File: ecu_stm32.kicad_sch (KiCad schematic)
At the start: 46 parts, among them J16 USB-C, J17 ARM Cortex Debug, Y2 16MHz

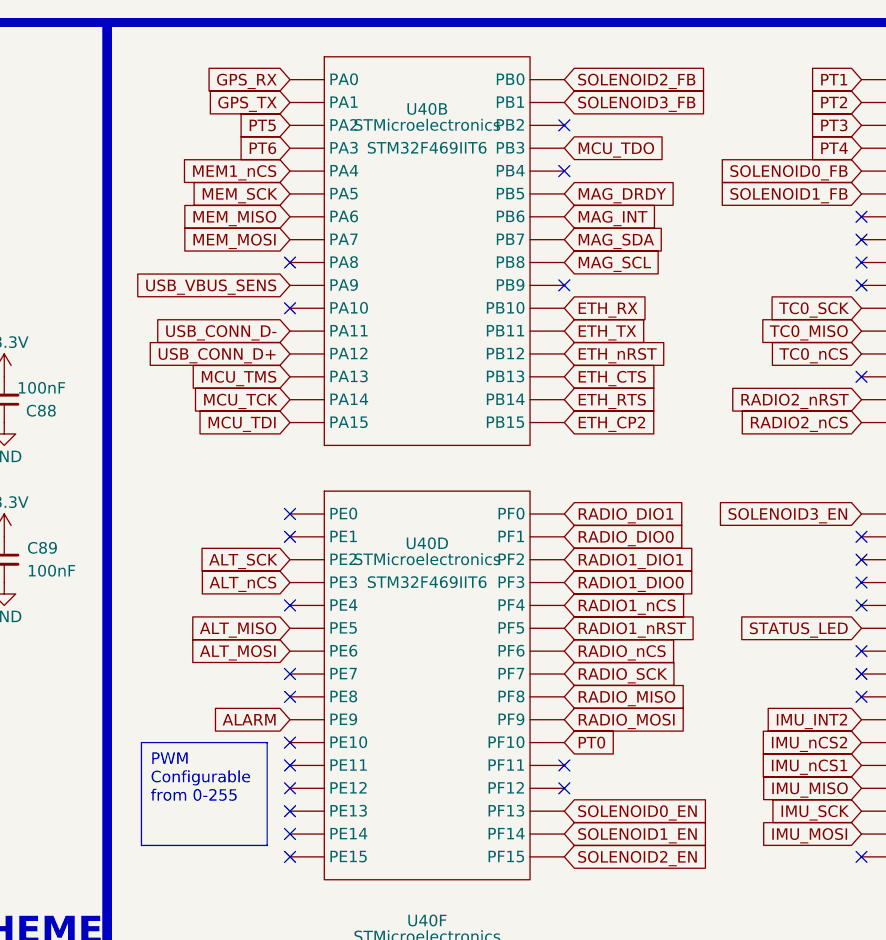
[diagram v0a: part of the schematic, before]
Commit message: Finished
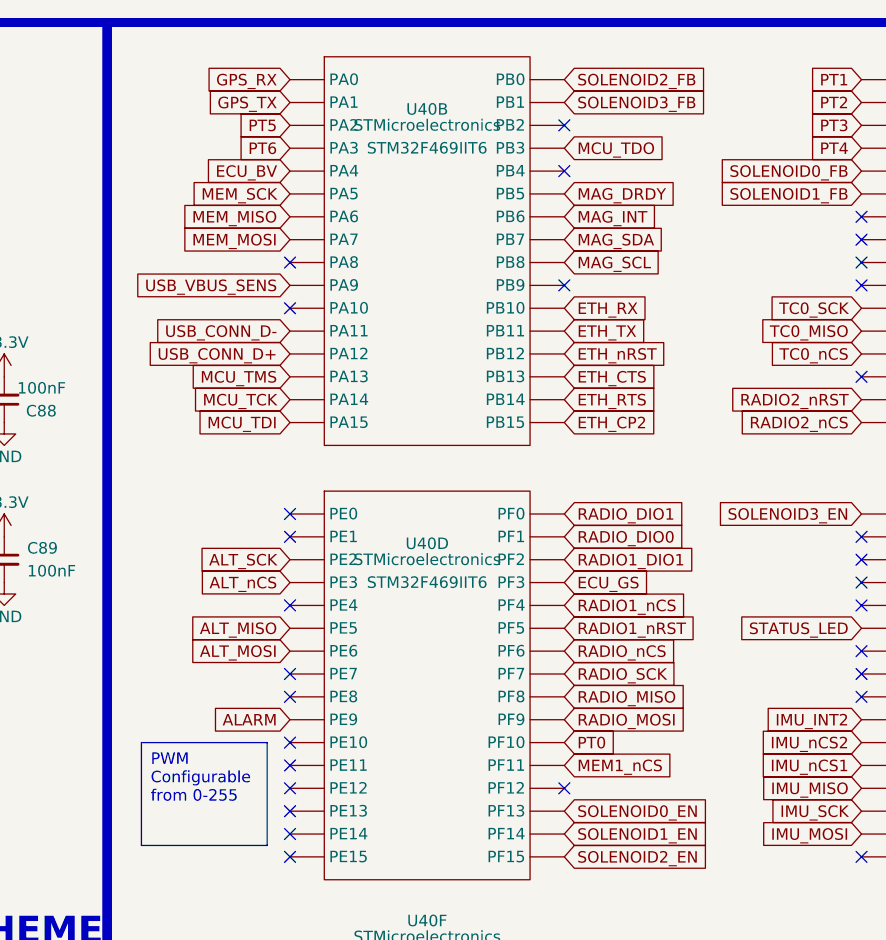
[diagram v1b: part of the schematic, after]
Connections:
- net MEM1_nCS: now also U40.59 (PF11); no longer U40.50 (PA4)
- net RADIO1_DIO0 renamed ECU_GS
- new net ECU_BV: U40.50 (PA4)
- no-connect marks 73 -> 72
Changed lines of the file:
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@@
 	)
 	(no_connect
-		(at 193.04 96.52)
-	)
-	(no_connect
 		(at 162.56 86.36)
 	)
@@
 		)
 	)
+	(global_label "ECU_GS"
+		(shape input)
+		(at 193.04 76.2 0)
+		(fields_autoplaced yes)
+		(effects
+			(font
+				(size 1.27 1.27)
+			)
+			(justify left)
+		)
+		(property "Intersheetrefs" "${INTERSHEET_REFS}"
+			(at 203.2218 76.2 0)
+			(effects
+				(font
+					(size 1.27 1.27)
+				)
+				(justify left)
+				(hide yes)
+			)
+		)
+	)
 	(global_label "IMU_MOSI"
 		(shape input)
@@
 		)
 	)
+	(global_label "ECU_BV"
+		(shape input)
+		(at 162.56 30.48 180)
+		(fields_autoplaced yes)
+		(effects
+			(font
+				(size 1.27 1.27)
+			)
+			(justify right)
+		)
+		(property "Intersheetrefs" "${INTERSHEET_REFS}"
+			(at 152.4991 30.48 0)
+			(effects
+				(font
+					(size 1.27 1.27)
+				)
+				(justify right)
+				(hide yes)
+			)
+		)
+	)
 	(global_label "PT4"
 		(shape input)
@@
 		)
 	)
-	(global_label "RADIO1_DIO0"
-		(shape input)
-		(at 193.04 76.2 0)
-		(fields_autoplaced yes)
-		(effects
-			(font
-				(size 1.27 1.27)
-			)
-			(justify left)
-		)
-		(property "Intersheetrefs" "${INTERSHEET_REFS}"
-			(at 208.181 76.2 0)
-			(effects
-				(font
-					(size 1.27 1.27)
-				)
-				(justify left)
-				(hide yes)
-			)
-		)
-	)
 	(global_label "GPS_INT"
 		(shape input)
@@
 		)
 	)
-	(global_label "MEM1_nCS"
+	(global_label "GPS_TX"
 		(shape input)
-		(at 162.56 30.48 180)
+		(at 162.56 22.86 180)
 		(fields_autoplaced yes)
 		(effects
@@
 		)
 		(property "Intersheetrefs" "${INTERSHEET_REFS}"
-			(at 149.7174 30.48 0)
+			(at 152.6806 22.86 0)
 			(effects
 				(font
@@
 		)
 	)
-	(global_label "GPS_TX"
+	(global_label "RADIO_MISO"
 		(shape input)
-		(at 162.56 22.86 180)
+		(at 193.04 88.9 0)
 		(fields_autoplaced yes)
 		(effects
@@
 				(size 1.27 1.27)
 			)
-			(justify right)
+			(justify left)
 		)
 		(property "Intersheetrefs" "${INTERSHEET_REFS}"
-			(at 152.6806 22.86 0)
+			(at 207.0735 88.9 0)
 			(effects
 				(font
 					(size 1.27 1.27)
 				)
-				(justify right)
+				(justify left)
 				(hide yes)
 			)
 		)
 	)
-	(global_label "RADIO_MISO"
+	(global_label "MEM1_nCS"
 		(shape input)
-		(at 193.04 88.9 0)
+		(at 193.04 96.52 0)
 		(fields_autoplaced yes)
 		(effects
@@
 		)
 		(property "Intersheetrefs" "${INTERSHEET_REFS}"
-			(at 207.0735 88.9 0)
+			(at 205.8826 96.52 0)
 			(effects
 				(font
